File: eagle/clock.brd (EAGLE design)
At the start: 160 x 100 mm, 55 parts, among them CN1 ARDUINO_SHIELDNO_SILK, IC1 TPS55330TRE, IC2 TCS3472FN, Q1 BC817-40SMD, Q2 SUD50P04-13L

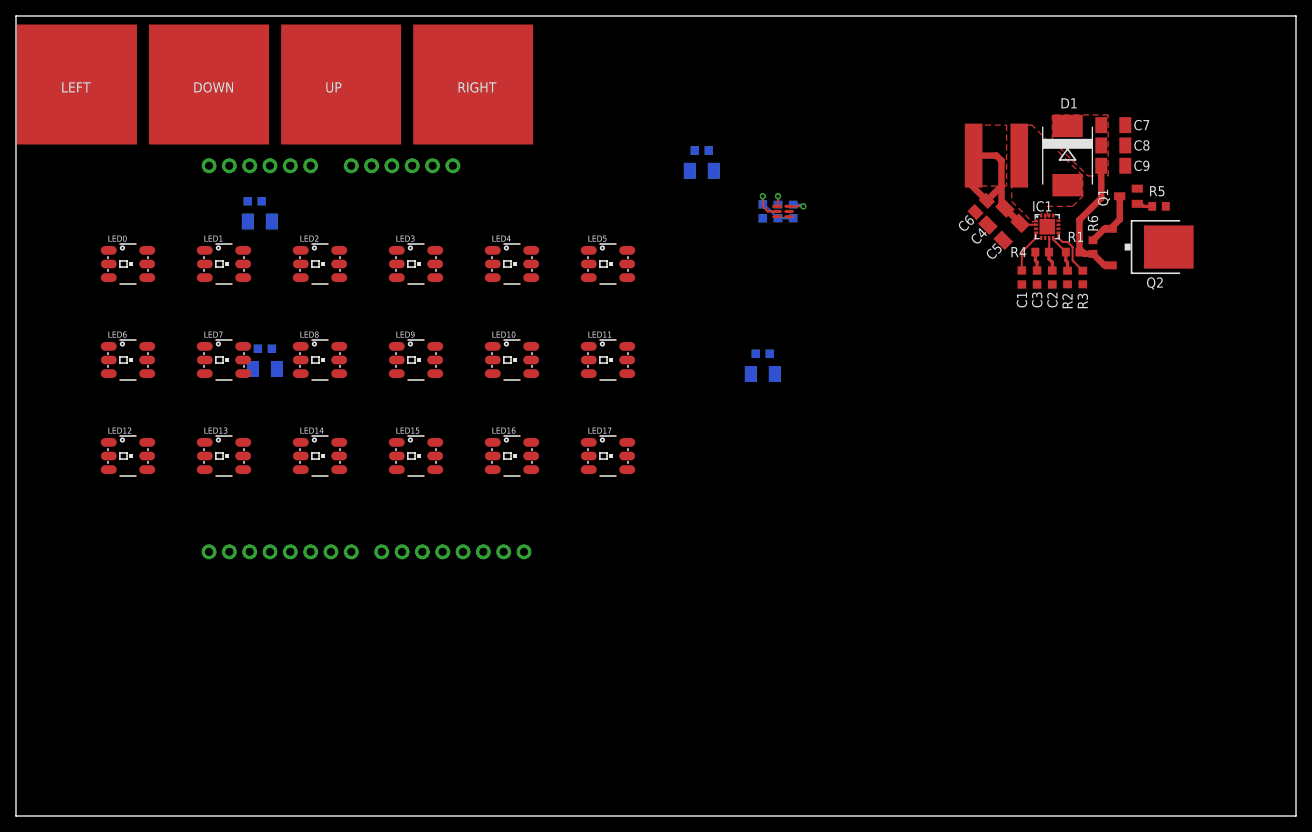
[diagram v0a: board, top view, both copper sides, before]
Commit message: Almost finished layout
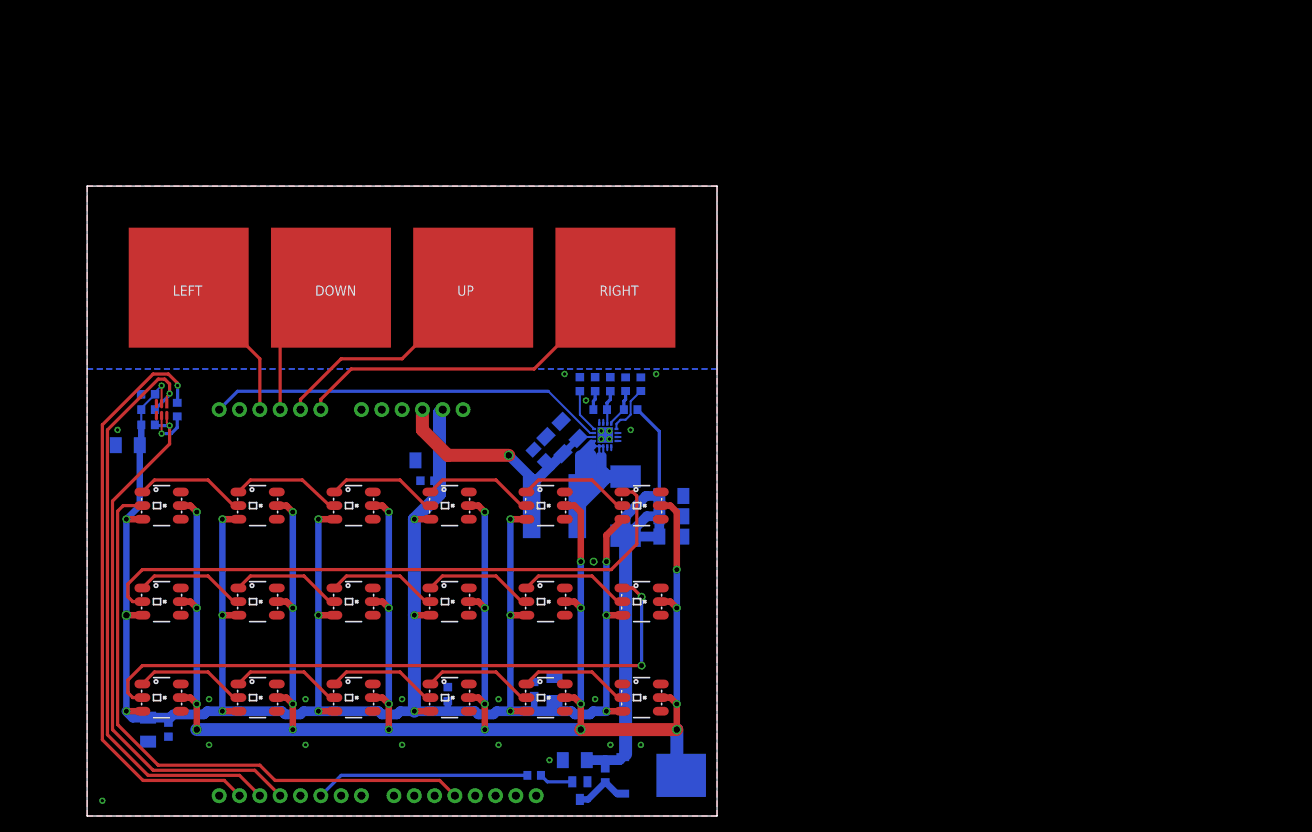
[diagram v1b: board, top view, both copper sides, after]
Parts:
- added C19: 10uF, rcl:C1206K
- added R9: 1k, rcl:R0603
- moved R5 105.6 mm to (64.8, 5.08), flipped to the bottom
- moved Q1 101.1 mm to (70.5, 3.17), flipped to the bottom, turned to 180 degrees
- moved R6 89.9 mm to (73.7, 5.08), flipped to the bottom, turned to 270 degrees
- moved Q2 89.9 mm to (80.6, 5.08), flipped to the bottom, turned to 90 degrees
- moved R7 84.9 mm to (16.5, 48.9), turned to 0 degrees
- moved R8 82.5 mm to (16.5, 50.8), turned to 0 degrees
- moved IC2 81.5 mm to (18.2, 50.8), turned to 270 degrees
- moved C10 80.2 mm to (16.5, 52.7), turned to 0 degrees
- moved C18 79.9 mm to (14.0, 46.4)
- moved C7 75.5 mm to (81.9, 34.9), flipped to the bottom, turned to 180 degrees
- moved C8 72.1 mm to (81.9, 37.5), flipped to the bottom, turned to 180 degrees
- moved D1 70.5 mm to (76.2, 38.7), flipped to the bottom, turned to 90 degrees
- moved L1 70.5 mm to (67.3, 38.7), flipped to the bottom, turned to 180 degrees
- moved C13 70.5 mm to (64.8, 15.9), turned to 90 degrees
- moved C9 69.0 mm to (81.9, 40.0), flipped to the bottom, turned to 180 degrees
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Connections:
- new net N$6: CN1.TX, R9.1
- net GND: now also C19.2
- net LIGHT-INT: now also R9.2; no longer CN1.D7
- net PWR-EN: now also CN1.A5; no longer CN1.D9
- net SMPSU-OUTPUT: now also C19.1
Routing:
- net 3.3V: track 9.12 -> 282.4 mm, vias 1 -> 19
- net 5V: track 0.00 -> 271.1 mm, vias 0 -> 24
- net N$25: track 0.00 -> 80.0 mm, vias 0 -> 2
- net N$19: track 0.00 -> 77.3 mm
- net LED-DATA: track 0.00 -> 75.9 mm
- net N$6: track 0.00 -> 74.4 mm, vias 0 -> 1
- net SCL: track 2.36 -> 76.3 mm
- net SDA: track 3.16 -> 68.6 mm
- net SMPSU-OUTPUT: track 16.5 -> 67.8 mm
- net PWR-EN: track 0.00 -> 50.0 mm
- net N$4: track 0.00 -> 43.9 mm
- net SW: track 0.00 -> 31.2 mm
- net N$3: track 0.00 -> 28.6 mm
- net LED-PWM: track 0.00 -> 26.9 mm
- net N$1: track 0.00 -> 18.9 mm
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- added copper zone on layer 1, net GND
- added copper zone on layer 16, net GND
- removed copper zone on layer 1, net SMPSU-OUTPUT
- removed copper zone on layer 1, net SW
- removed copper zone on layer 1, net V_BATT
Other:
- board size 160 x 100 mm -> 78.7 x 78.7 mm
